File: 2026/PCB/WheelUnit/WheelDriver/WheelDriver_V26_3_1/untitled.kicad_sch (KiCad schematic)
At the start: 56 parts, among them SW3 SW_MEC_5E

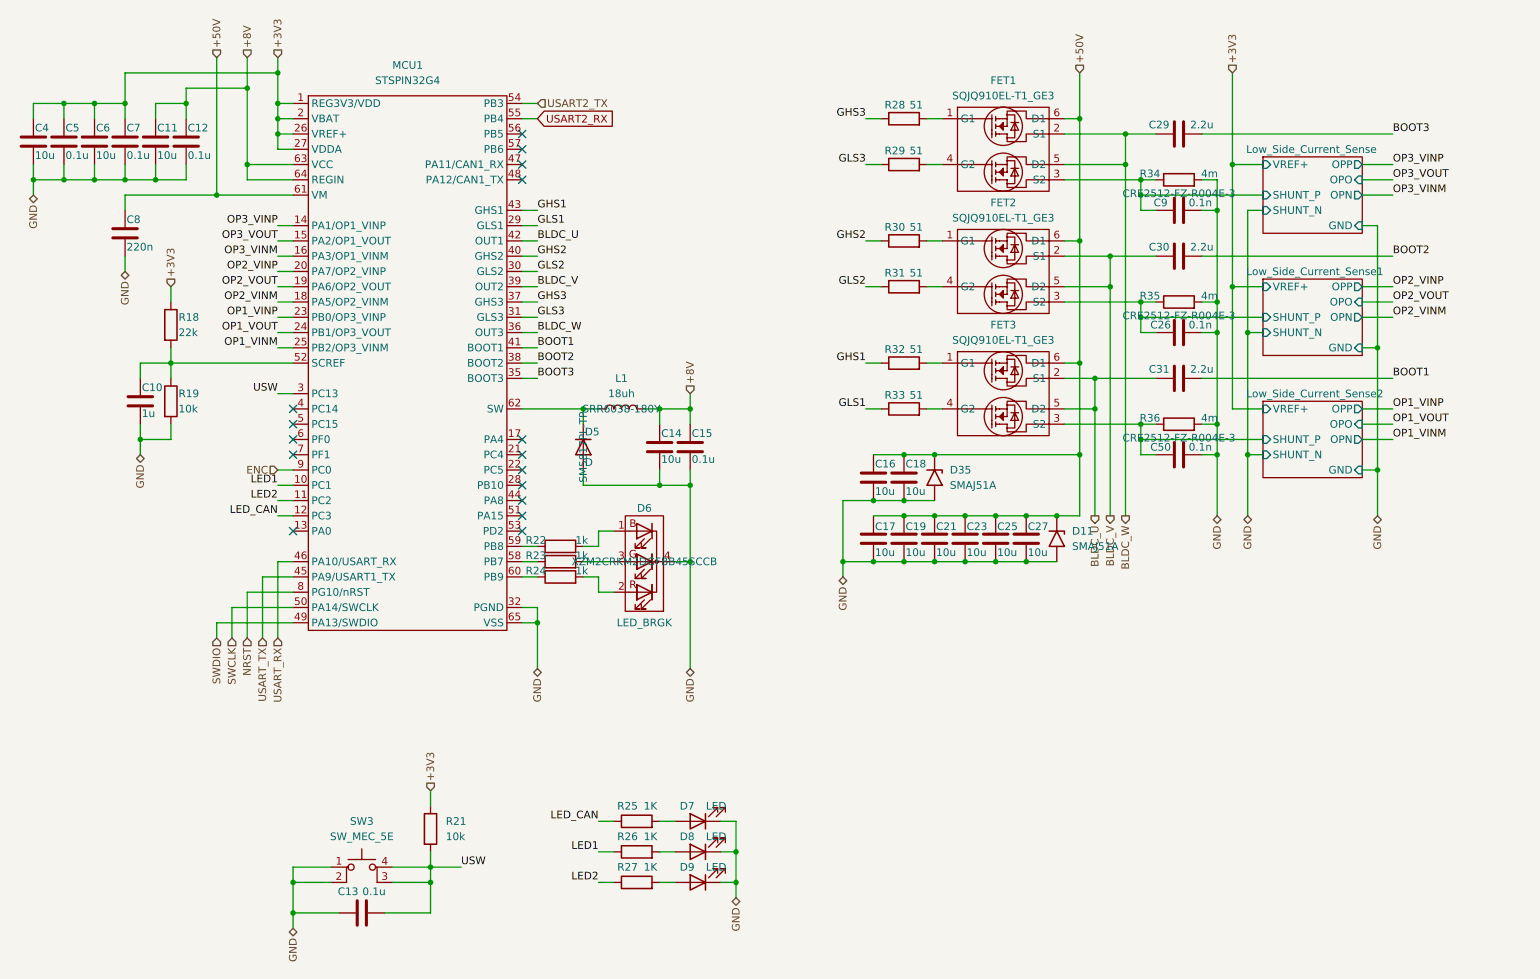
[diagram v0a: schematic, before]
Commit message: STSPIN32G4回り修正
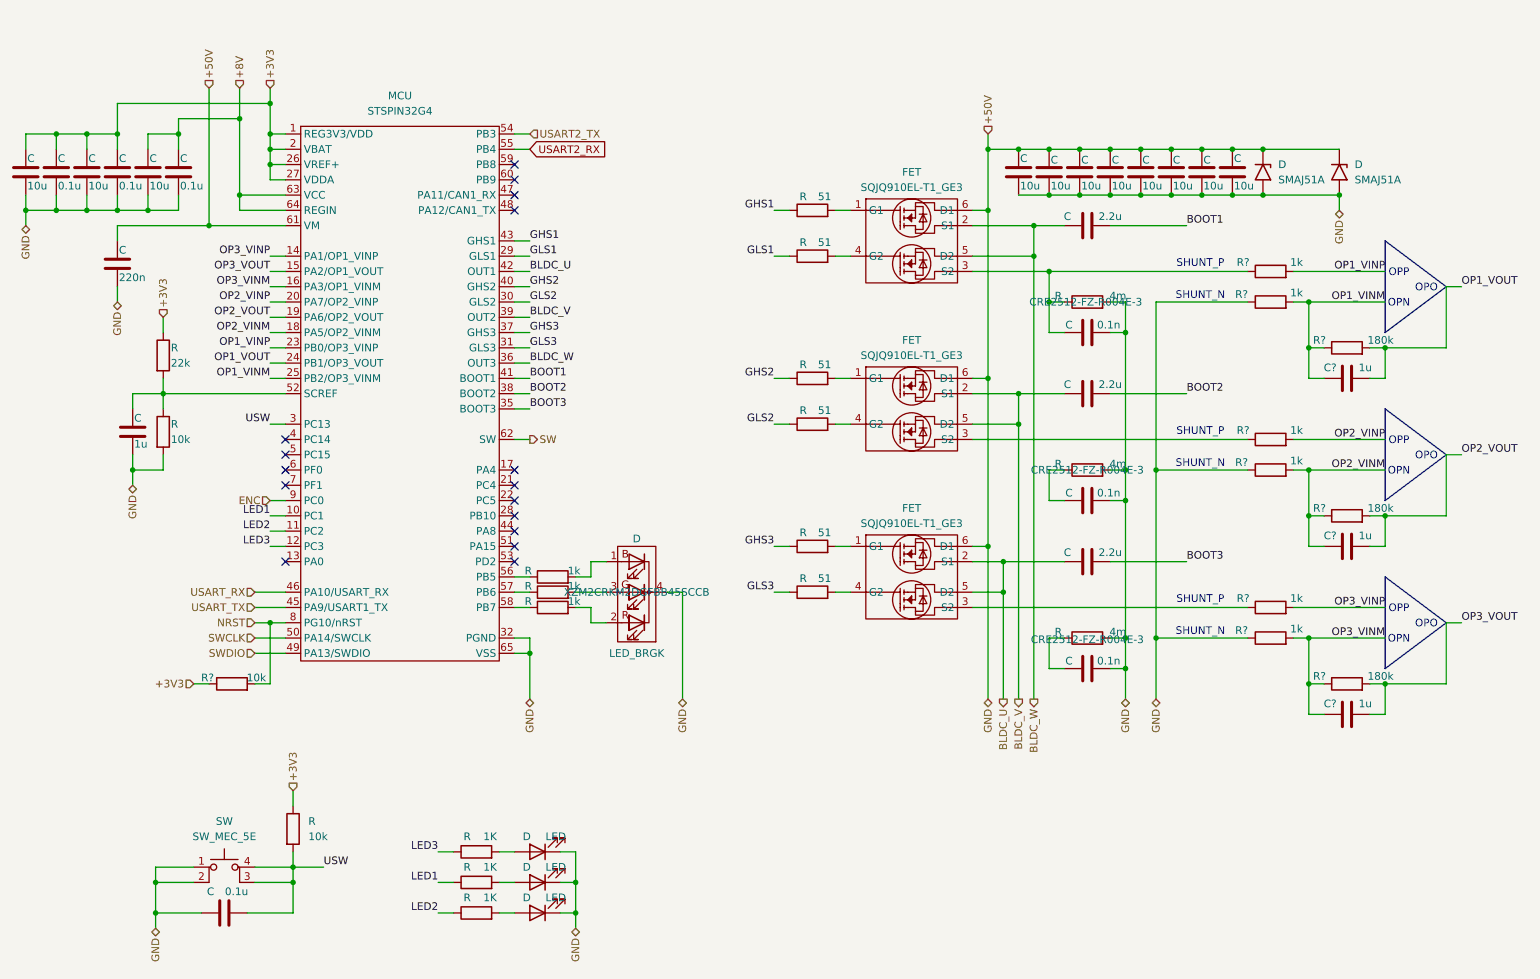
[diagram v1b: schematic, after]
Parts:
- removed C14: 10u, Capacitor_SMD:C_0603_1608Metric_Pad1.08x0.95mm_HandSolder, symbol Device:C
- removed C15: 0.1u, Capacitor_SMD:C_0603_1608Metric_Pad1.08x0.95mm_HandSolder, symbol Device:C
- removed D5: D, Diode_SMD:D_SOD-123F, symbol Device:D
- removed L1: 18uh, WheelUnit_LIB_FTP:IND_SRR6038-180Y, symbol Device:L
- added C? (x3): 1u, Capacitor_SMD:C_0402_1005Metric_Pad0.74x0.62mm_HandSolder, symbol Device:C
- added R? (x6): 1k, Resistor_SMD:R_0402_1005Metric_Pad0.72x0.64mm_HandSolder, symbol Device:R
- added R? (x3): 180k, Resistor_SMD:R_0402_1005Metric_Pad0.72x0.64mm_HandSolder, symbol Device:R
- added R?: 10k, Resistor_SMD:R_0402_1005Metric_Pad0.72x0.64mm_HandSolder, symbol Device:R
- renumbered C6 to C, C13 to C, C5 to C, C18 to C, C29 to C, C16 to C, C19 to C, C12 to C, C27 to C, C21 to C, C4 to C, C9 to C, C17 to C, C25 to C, C31 to C, C7 to C, C8 to C, C10 to C, C11 to C, C30 to C, C50 to C, C26 to C, C23 to C, D8 to D, D7 to D, D9 to D, D11 to D, D35 to D, D6 to D, FET3 to FET, FET1 to FET, FET2 to FET, MCU1 to MCU, R31 to R, R27 to R, R28 to R, R25 to R, R29 to R, R36 to R, R21 to R, R33 to R, R19 to R, R35 to R, R34 to R, R23 to R, R18 to R, R22 to R, R26 to R, R30 to R, R32 to R, R24 to R, SW3 to SW
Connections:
- net GND is gone; now on net +50V: C.1, C.1, C.1, C.2, C.2, C.2, C.2, C.2, C.2, C.2, C.2, C.2, C.2, C.2, C.2, C.2, C.2, C.2, C.2, C.2, D.1 (K), D.1 (K), D.1 (K), D.2 (A2), D.2 (A2), D.4 (K), MCU.32 (PGND), MCU.65 (VSS), R.2, R.2, R.2, R.2, SW.1, SW.2
- net +3V3: now also R?.1
- net +50V: now also R?.1, R?.1, R?.1
- net BOOT1: now also C.2; no longer C.2
- net BOOT3: now also C.2; no longer C.2
- net GHS1: now also R.1; no longer R.1
- net GHS3: now also R.1; no longer R.1
- net GLS1: now also R.1; no longer R.1
- net GLS3: now also R.1; no longer R.1
- net NRST: now also R?.2
- net OP1_VINM: now also C?.2, R?.1, R?.2
- net OP1_VINP: now also R?.2
- net OP1_VOUT: now also C?.1, R?.2
- net OP2_VINM: now also C?.2, R?.1, R?.2
- net OP2_VINP: now also R?.2
- net OP2_VOUT: now also C?.1, R?.2
- net OP3_VINM: now also C?.2, R?.1, R?.2
- net OP3_VINP: now also R?.2
- net OP3_VOUT: now also C?.1, R?.2
- net SW: now reaches MCU.62 (SW)
- net at MCU.56 (PB5): now also R.1
- net at MCU.57 (PB6): now also R.1
- net at MCU.58 (PB7): now also R.1; no longer R.1
- net at MCU.59 (PB8): no longer R.1
- net at MCU.60 (PB9): no longer R.1
- net LED_CAN renamed LED3
- net Low_Side_Current_Sense/SHUNT_P: no longer names the net of C.2, FET.3 (S2), R.1
- net Low_Side_Current_Sense/SHUNT_P: now also R?.1
- net Low_Side_Current_Sense1/SHUNT_P: no longer names the net of C.2, R.1
- net Low_Side_Current_Sense1/SHUNT_P: no longer FET.3 (S2)
- net Low_Side_Current_Sense2/SHUNT_P: no longer names the net of C.2, R.1
- net Low_Side_Current_Sense2/SHUNT_P: no longer FET.3 (S2)
- new net: FET.3 (S2), R?.1 (x2)
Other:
- removed sheet Low_Side_Current_Sense
- removed sheet Low_Side_Current_Sense1
- removed sheet Low_Side_Current_Sense2
- note added: "OPN"
- note added: "OPO"
- note added: "OPP"
- note added: "SHUNT_N"
- note added: "SHUNT_P"
- moved on the sheet: C, D, FET, MCU, R, SW
